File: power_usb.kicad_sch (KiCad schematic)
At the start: 12 parts, among them J5 USB_C_Receptacle_USB2.0_16P, J6 BAT, U8 AMS1117-3.3

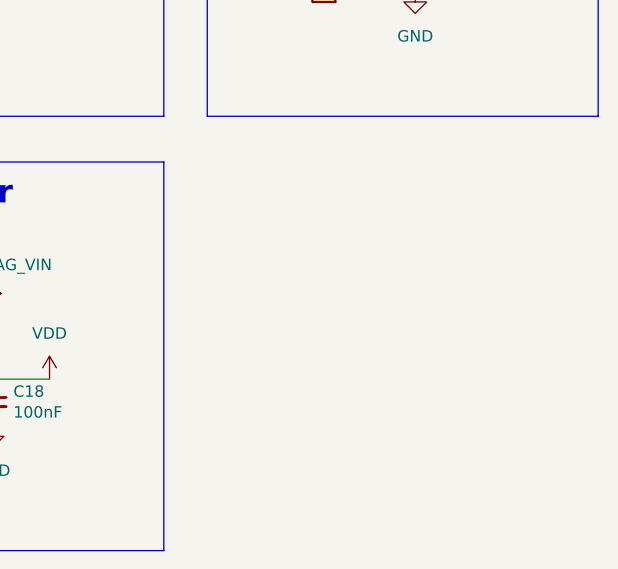
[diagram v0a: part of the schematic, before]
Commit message: Schematics: Add uSD card holder & VBAT sensing
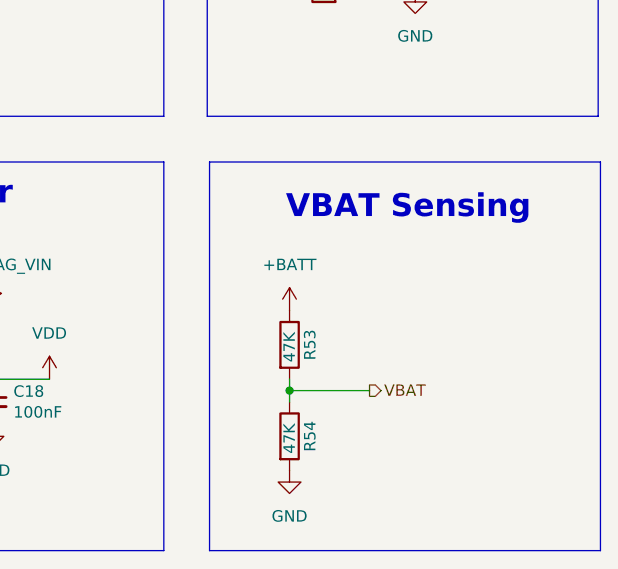
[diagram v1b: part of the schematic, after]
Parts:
- added R53, R54: 47K, Resistor_SMD:R_0402_1005Metric, symbol Device:R
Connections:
- net +BATT: now also R53.1
- net GND: now also R54.2
- new net VBAT: R53.2, R54.1
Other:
- note added: "VBAT Sensing"

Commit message: Schematics: Add accelerometer, drop VBAT sensing
Adding a cheap accelerometer to the boards, sacraficing the VBAT input
to make room for the /CS pin.
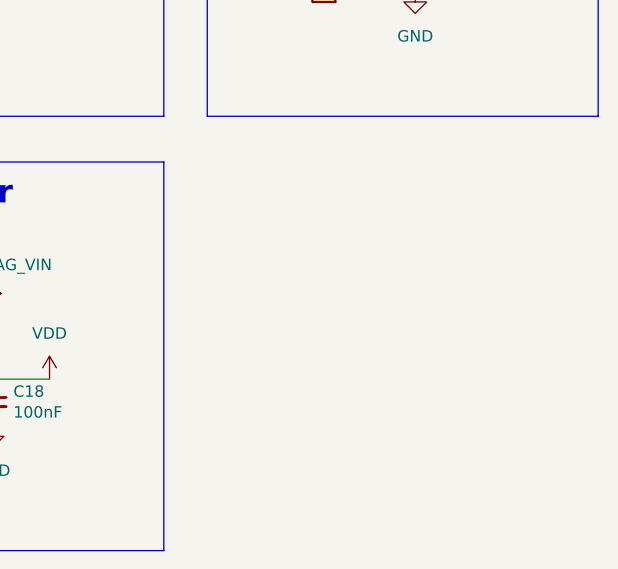
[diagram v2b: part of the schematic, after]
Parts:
- removed R53, R54: 47K, Resistor_SMD:R_0402_1005Metric, symbol Device:R
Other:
- note removed: "VBAT Sensing"
